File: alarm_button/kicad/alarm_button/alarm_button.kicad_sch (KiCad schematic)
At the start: 5 parts, among them SW1 SW_Push

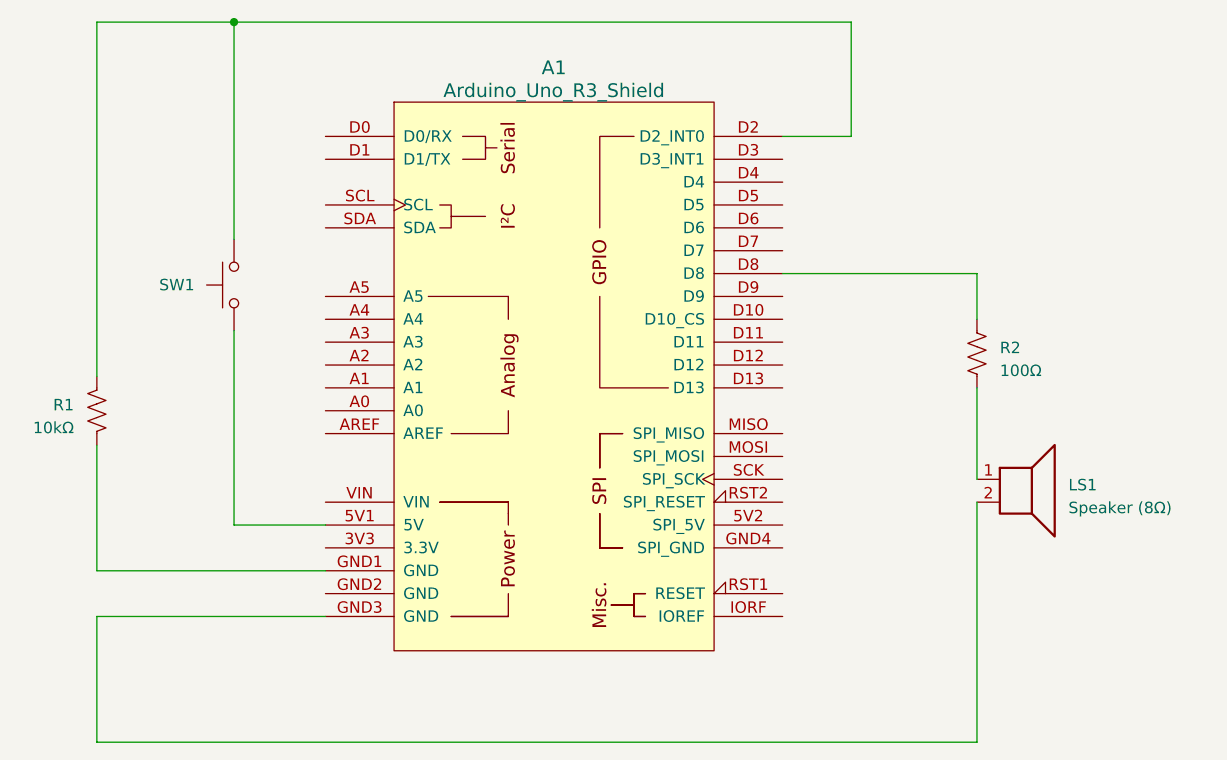
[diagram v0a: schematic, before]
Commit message: Use default Arduino UNO R3 symbol
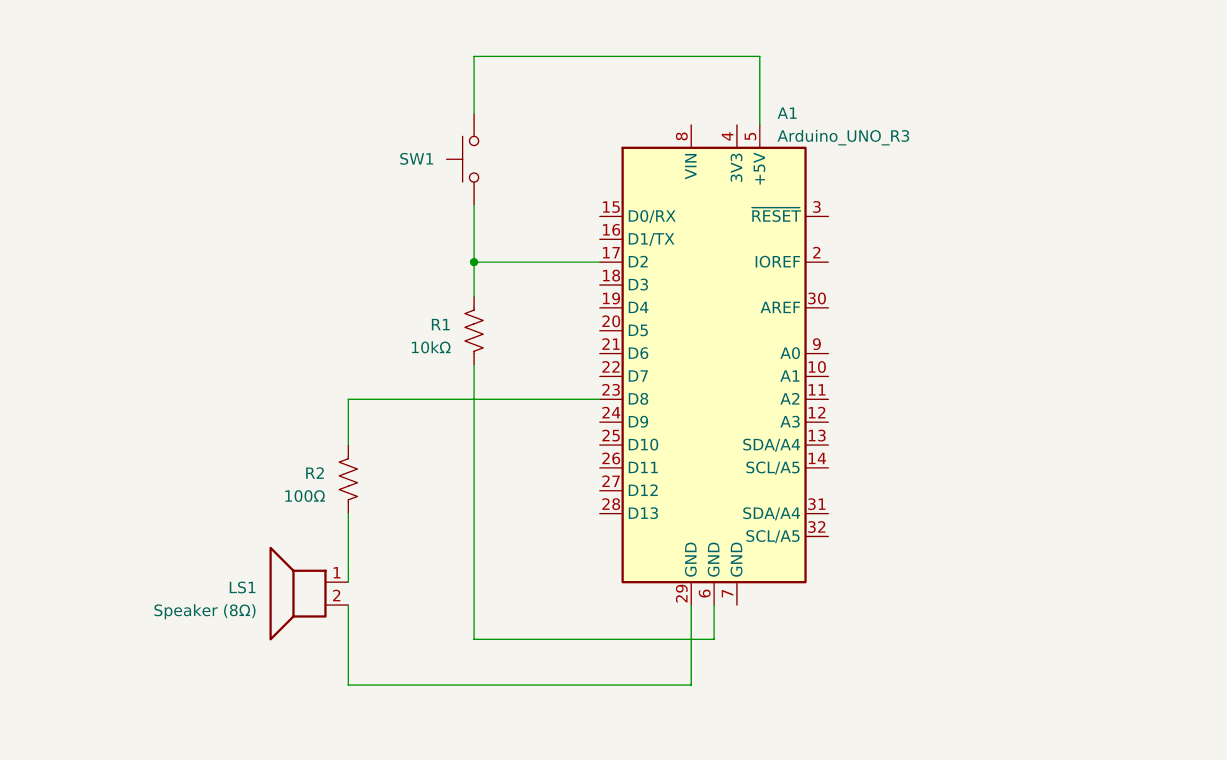
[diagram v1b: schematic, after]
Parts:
- removed A1: Arduino_Uno_R3_Shield, PCM_arduino-library:Arduino_Uno_R3_Shield, symbol PCM_arduino-library:Arduino_Uno_R3_Shield
- added A1: Arduino_UNO_R3, Module:Arduino_UNO_R3, symbol MCU_Module:Arduino_UNO_R3
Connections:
- net at SW1.2: now also R1.1, A1.17 (D2)
- net at SW1.1: now also A1.5 (+5V); no longer R1.1
- net at R2.1: now also A1.23 (D8)
- net at R1.2: now also A1.6 (GND)
- net at LS1.2: now also A1.29 (GND)
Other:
- moved on the sheet: LS1, R1, R2, SW1
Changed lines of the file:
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@@
     (title "Alarm Button")
   )
-  (junction (at 66.04 20.32) (diameter 0) (color 0 0 0 0)
+  (junction (at 92.71 46.99) (diameter 0) (color 0 0 0 0)
   )
-  (wire (pts (xy 127 48.26) (xy 148.59 48.26))
+  (wire (pts (xy 124.46 24.13) (xy 92.71 24.13))
     (stroke (width 0) (type default))
   )
-  (wire (pts (xy 50.8 59.69) (xy 50.8 20.32))
+  (wire (pts (xy 92.71 40.64) (xy 92.71 46.99))
     (stroke (width 0) (type default))
   )
-  (wire (pts (xy 50.8 20.32) (xy 66.04 20.32))
+  (wire (pts (xy 78.74 93.98) (xy 116.84 93.98))
     (stroke (width 0) (type default))
   )
-  (wire (pts (xy 148.59 48.26) (xy 148.59 53.34))
+  (wire (pts (xy 92.71 24.13) (xy 92.71 30.48))
     (stroke (width 0) (type default))
   )
-  (wire (pts (xy 50.8 100.33) (xy 50.8 86.36))
+  (wire (pts (xy 78.74 62.23) (xy 78.74 67.31))
     (stroke (width 0) (type default))
   )
-  (wire (pts (xy 50.8 81.28) (xy 76.2 81.28))
+  (wire (pts (xy 124.46 31.75) (xy 124.46 24.13))
     (stroke (width 0) (type default))
   )
-  (wire (pts (xy 66.04 76.2) (xy 66.04 54.61))
+  (wire (pts (xy 106.68 62.23) (xy 78.74 62.23))
     (stroke (width 0) (type default))
   )
-  (wire (pts (xy 66.04 44.45) (xy 66.04 20.32))
+  (wire (pts (xy 119.38 88.9) (xy 119.38 85.09))
     (stroke (width 0) (type default))
   )
-  (wire (pts (xy 76.2 76.2) (xy 66.04 76.2))
+  (wire (pts (xy 92.71 88.9) (xy 119.38 88.9))
     (stroke (width 0) (type default))
   )
-  (wire (pts (xy 66.04 20.32) (xy 134.62 20.32))
+  (wire (pts (xy 92.71 46.99) (xy 92.71 50.8))
     (stroke (width 0) (type default))
   )
-  (wire (pts (xy 148.59 73.66) (xy 148.59 100.33))
+  (wire (pts (xy 78.74 74.93) (xy 78.74 82.55))
     (stroke (width 0) (type default))
   )
-  (wire (pts (xy 148.59 100.33) (xy 50.8 100.33))
+  (wire (pts (xy 116.84 93.98) (xy 116.84 85.09))
     (stroke (width 0) (type default))
   )
-  (wire (pts (xy 50.8 86.36) (xy 76.2 86.36))
+  (wire (pts (xy 92.71 58.42) (xy 92.71 88.9))
     (stroke (width 0) (type default))
   )
-  (wire (pts (xy 134.62 20.32) (xy 134.62 33.02))
+  (wire (pts (xy 92.71 46.99) (xy 106.68 46.99))
     (stroke (width 0) (type default))
   )
-  (wire (pts (xy 50.8 67.31) (xy 50.8 81.28))
+  (wire (pts (xy 78.74 85.09) (xy 78.74 93.98))
     (stroke (width 0) (type default))
   )
-  (wire (pts (xy 134.62 33.02) (xy 127 33.02))
-    (stroke (width 0) (type default))
-  )
-  (wire (pts (xy 148.59 60.96) (xy 148.59 71.12))
-    (stroke (width 0) (type default))
-  )
-  (symbol (lib_id "PCM_arduino-library:Arduino_Uno_R3_Shield") (at 101.6 59.69 0) (unit 1)
+  (symbol (lib_id "MCU_Module:Arduino_UNO_R3") (at 119.38 57.15 0) (unit 1)
     (in_bom yes) (on_board yes) (dnp no) (fields_autoplaced)
-    (property "Reference" "A1" (at 101.6 25.4 0)
-      (effects (font (size 1.524 1.524)))
+    (property "Reference" "A1" (at 126.4159 30.48 0)
+      (effects (font (size 1.27 1.27)) (justify left))
     )
-    (property "Value" "Arduino_Uno_R3_Shield" (at 101.6 27.94 0)
-      (effects (font (size 1.524 1.524)))
+    (property "Value" "Arduino_UNO_R3" (at 126.4159 33.02 0)
+      (effects (font (size 1.27 1.27)) (justify left))
     )
-    (property "Footprint" "PCM_arduino-library:Arduino_Uno_R3_Shield" (at 101.6 97.79 0)
-      (effects (font (size 1.524 1.524)) hide)
+    (property "Footprint" "Module:Arduino_UNO_R3" (at 119.38 57.15 0)
+      (effects (font (size 1.27 1.27) italic) hide)
     )
-    (property "Datasheet" "https://docs.arduino.cc/hardware/uno-rev3" (at 101.6 93.98 0)
-      (effects (font (size 1.524 1.524)) hide)
+    (property "Datasheet" "https://www.arduino.cc/en/Main/arduinoBoardUno" (at 119.38 57.15 0)
+      (effects (font (size 1.27 1.27)) hide)
     )
-    (pin "3V3")
-    (pin "5V1")
-    (pin "5V2")
-    (pin "A0")
-    (pin "A1")
-    (pin "A2")
-    (pin "A3")
-    (pin "A4")
-    (pin "A5")
-    (pin "AREF")
-    (pin "D0")
-    (pin "D1")
-    (pin "D10")
-    (pin "D11")
-    (pin "D12")
-    (pin "D13")
-    (pin "D2")
-    (pin "D3")
-    (pin "D4")
-    (pin "D5")
-    (pin "D6")
-    (pin "D7")
-    (pin "D8")
-    (pin "D9")
-    (pin "GND1")
-    (pin "GND2")
-    (pin "GND3")
-    (pin "GND4")
-    (pin "IORF")
-    (pin "MISO")
-    (pin "MOSI")
-    (pin "RST1")
-    (pin "RST2")
-    (pin "SCK")
-    (pin "SCL")
-    (pin "SDA")
-    (pin "VIN")
+    (pin "1")
+    (pin "10")
+    (pin "11")
+    (pin "12")
+    (pin "13")
+    (pin "14")
+    (pin "15")
+    (pin "16")
+    (pin "17")
+    (pin "18")
+    (pin "19")
+    (pin "2")
+    (pin "20")
+    (pin "21")
+    (pin "22")
+    (pin "23")
+    (pin "24")
+    (pin "25")
+    (pin "26")
+    (pin "27")
+    (pin "28")
+    (pin "29")
+    (pin "3")
+    (pin "30")
+    (pin "31")
+    (pin "32")
+    (pin "4")
+    (pin "5")
+    (pin "6")
+    (pin "7")
+    (pin "8")
+    (pin "9")
     (instances
       (project "alarm_button"
@@
     )
   )
-  (symbol (lib_id "Device:Speaker") (at 153.67 71.12 0) (unit 1)
-    (in_bom yes) (on_board yes) (dnp no) (fields_autoplaced)
-    (property "Reference" "LS1" (at 158.75 71.755 0)
+  (symbol (lib_id "Device:Speaker") (at 73.66 82.55 0) (mirror y) (unit 1)
+    (in_bom yes) (on_board yes) (dnp no)
+    (property "Reference" "LS1" (at 68.58 83.185 0)
       (effects (font (size 1.27 1.27)) (justify left))
     )
-    (property "Value" "Speaker (8Ω)" (at 158.75 74.295 0)
+    (property "Value" "Speaker (8Ω)" (at 68.58 85.725 0)
       (effects (font (size 1.27 1.27)) (justify left))
     )
-    (property "Footprint" "" (at 153.67 76.2 0)
+    (property "Footprint" "" (at 73.66 87.63 0)
       (effects (font (size 1.27 1.27)) hide)
     )
-    (property "Datasheet" "~" (at 153.416 72.39 0)
+    (property "Datasheet" "~" (at 73.914 83.82 0)
       (effects (font (size 1.27 1.27)) hide)
     )
@@
     )
   )
-  (symbol (lib_id "Device:R_US") (at 50.8 63.5 0) (mirror y) (unit 1)
+  (symbol (lib_id "Device:R_US") (at 92.71 54.61 0) (mirror y) (unit 1)
     (in_bom yes) (on_board yes) (dnp no)
-    (property "Reference" "R1" (at 48.26 62.865 0)
+    (property "Reference" "R1" (at 90.17 53.975 0)
       (effects (font (size 1.27 1.27)) (justify left))
     )
-    (property "Value" "10kΩ" (at 48.26 65.405 0)
+    (property "Value" "10kΩ" (at 90.17 56.515 0)
       (effects (font (size 1.27 1.27)) (justify left))
     )
-    (property "Footprint" "" (at 49.784 63.754 90)
+    (property "Footprint" "" (at 91.694 54.864 90)
       (effects (font (size 1.27 1.27)) hide)
     )
-    (property "Datasheet" "~" (at 50.8 63.5 0)
+    (property "Datasheet" "~" (at 92.71 54.61 0)
       (effects (font (size 1.27 1.27)) hide)
     )
@@
     )
   )
-  (symbol (lib_id "Switch:SW_Push") (at 66.04 49.53 90) (mirror x) (unit 1)
+  (symbol (lib_id "Switch:SW_Push") (at 92.71 35.56 90) (mirror x) (unit 1)
     (in_bom yes) (on_board yes) (dnp no)
-    (property "Reference" "SW1" (at 59.69 49.53 90)
+    (property "Reference" "SW1" (at 86.36 35.56 90)
       (effects (font (size 1.27 1.27)))
     )
-    (property "Value" "SW_Push" (at 60.96 50.8 90)
+    (property "Value" "SW_Push" (at 87.63 36.83 90)
       (effects (font (size 1.27 1.27)) hide)
     )
-    (property "Footprint" "" (at 60.96 49.53 0)
+    (property "Footprint" "" (at 87.63 35.56 0)
       (effects (font (size 1.27 1.27)) hide)
     )
-    (property "Datasheet" "~" (at 60.96 49.53 0)
+    (property "Datasheet" "~" (at 87.63 35.56 0)
       (effects (font (size 1.27 1.27)) hide)
     )
@@
     )
   )
-  (symbol (lib_id "Device:R_US") (at 148.59 57.15 0) (unit 1)
+  (symbol (lib_id "Device:R_US") (at 78.74 71.12 0) (mirror y) (unit 1)
     (in_bom yes) (on_board yes) (dnp no)
-    (property "Reference" "R2" (at 151.13 56.515 0)
+    (property "Reference" "R2" (at 76.2 70.485 0)
       (effects (font (size 1.27 1.27)) (justify left))
     )
-    (property "Value" "100Ω" (at 151.13 59.055 0)
+    (property "Value" "100Ω" (at 76.2 73.025 0)
       (effects (font (size 1.27 1.27)) (justify left))
     )
-    (property "Footprint" "" (at 149.606 57.404 90)
+    (property "Footprint" "" (at 77.724 71.374 90)
       (effects (font (size 1.27 1.27)) hide)
     )
-    (property "Datasheet" "~" (at 148.59 57.15 0)
+    (property "Datasheet" "~" (at 78.74 71.12 0)
       (effects (font (size 1.27 1.27)) hide)
     )
